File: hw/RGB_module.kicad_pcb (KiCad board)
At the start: 2 copper layers, 30 x 10 mm, 11 parts, among them J1 Conn_01x04, J2 Conn_01x04, J3 Conn_01x03, U1 ZSCS-2016C-08D-Z4

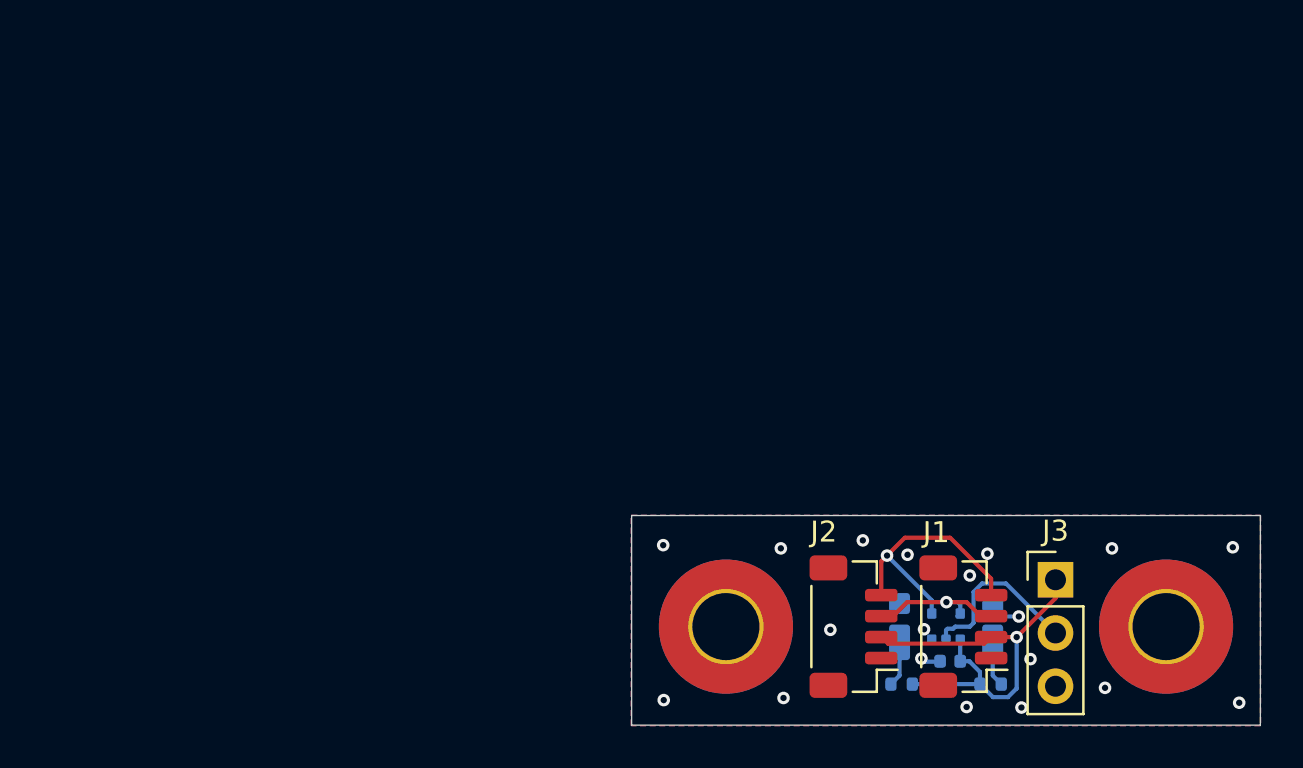
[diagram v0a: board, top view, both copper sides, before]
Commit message: board_v2
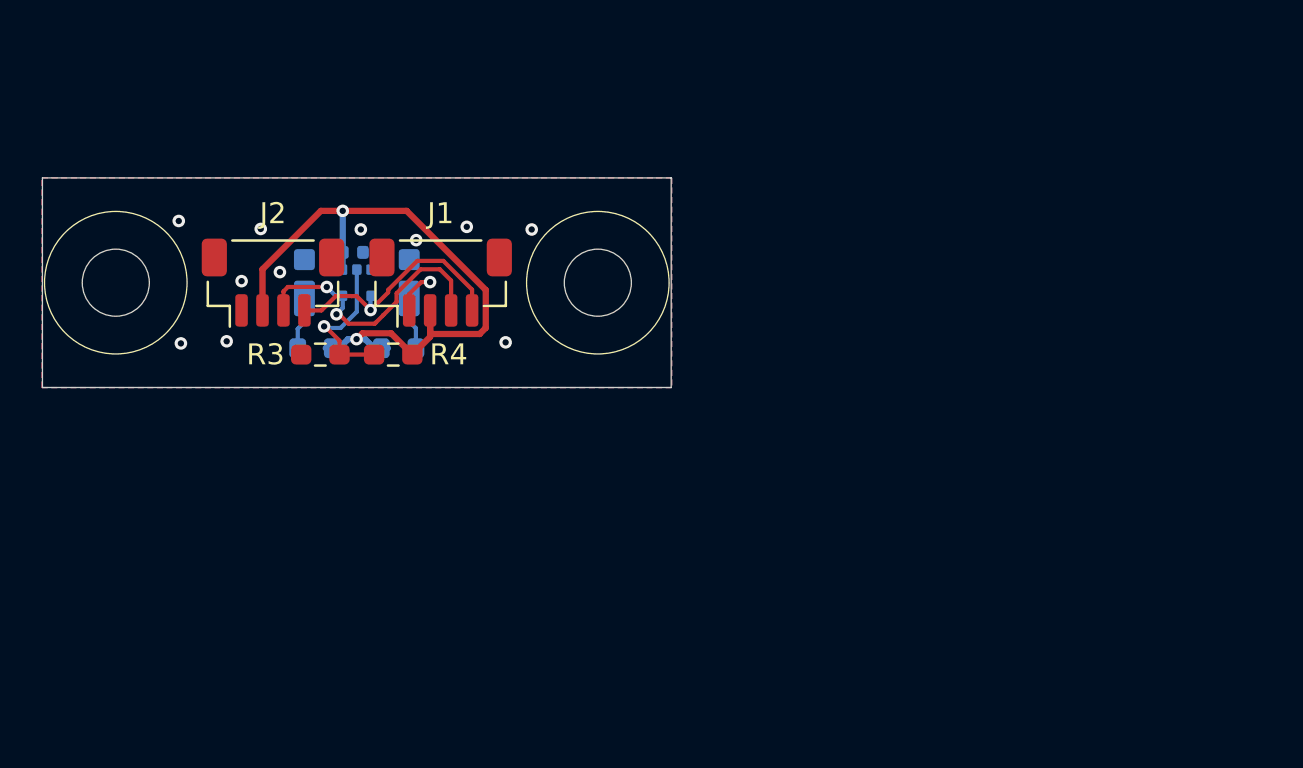
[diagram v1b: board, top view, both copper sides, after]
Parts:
- removed H1, H2: MountingHole, MountingHole:MountingHole_3.2mm_M3_Pad_TopBottom
- removed J3: Conn_01x03, Connector_PinHeader_2.54mm:PinHeader_1x03_P2.54mm_Vertical
- added R3: 0, Resistor_SMD:R_0603_1608Metric_Pad0.98x0.95mm_HandSolder, F.Cu at (45.1, 31.4)
- added R4: 100k, Resistor_SMD:R_0603_1608Metric_Pad0.98x0.95mm_HandSolder, F.Cu at (48.5, 31.4)
- R1, R2: value 8 -> 33; footprint Resistor_SMD:R_0402_1005Metric -> Resistor_SMD:R_0603_1608Metric
- moved C1 34.5 mm to (46.6, 26.5), turned to 0 degrees
- moved D1 32.8 mm to (44.3, 27.9)
- moved U1 32.6 mm to (46.8, 27.9), turned to 90 degrees
- moved R2 32.5 mm to (48.8, 31.1)
- moved D2 32.3 mm to (49.3, 27.9)
- moved R1 32.3 mm to (44.8, 31.1)
- moved J2 32.2 mm to (42.8, 27.9), turned to 0 degrees
- moved J1 29.9 mm to (50.8, 27.9), turned to 0 degrees
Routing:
- net +3.3V: track 20.9 -> 32.8 mm, vias 1 -> 2
- net SDA: track 7.12 -> 13.6 mm, vias 1 -> 2
- net Net-(U1-ADDR): track 8.44 -> 7.26 mm, vias 0 -> 1
- net SCL: track 12.6 -> 11.9 mm
- net GND: track 2.65 -> 2.01 mm, vias 19 -> 12
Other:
- outline, holes or cut-outs redrawn

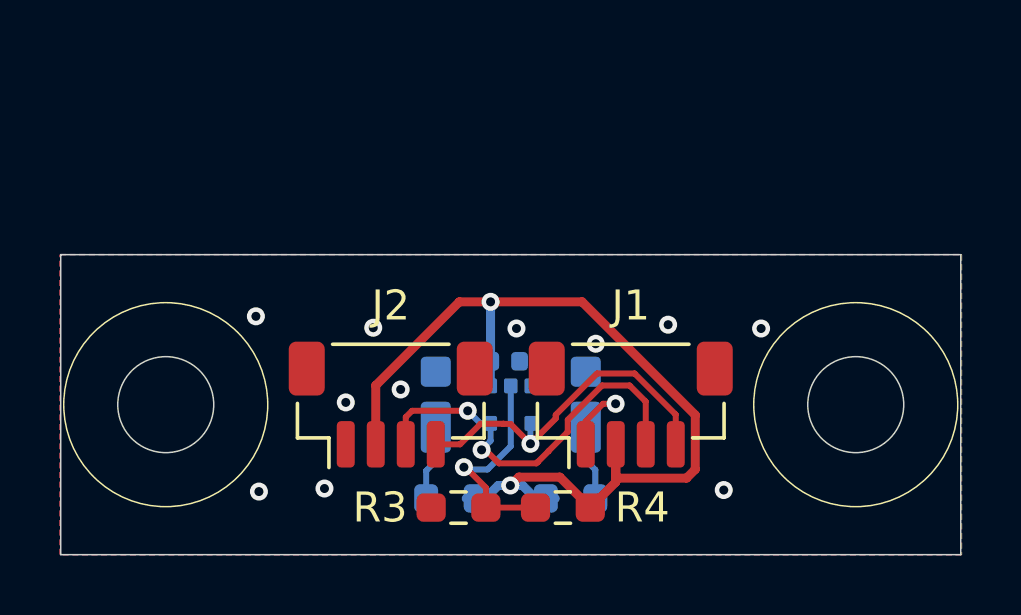
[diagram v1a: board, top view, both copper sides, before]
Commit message: board_v3
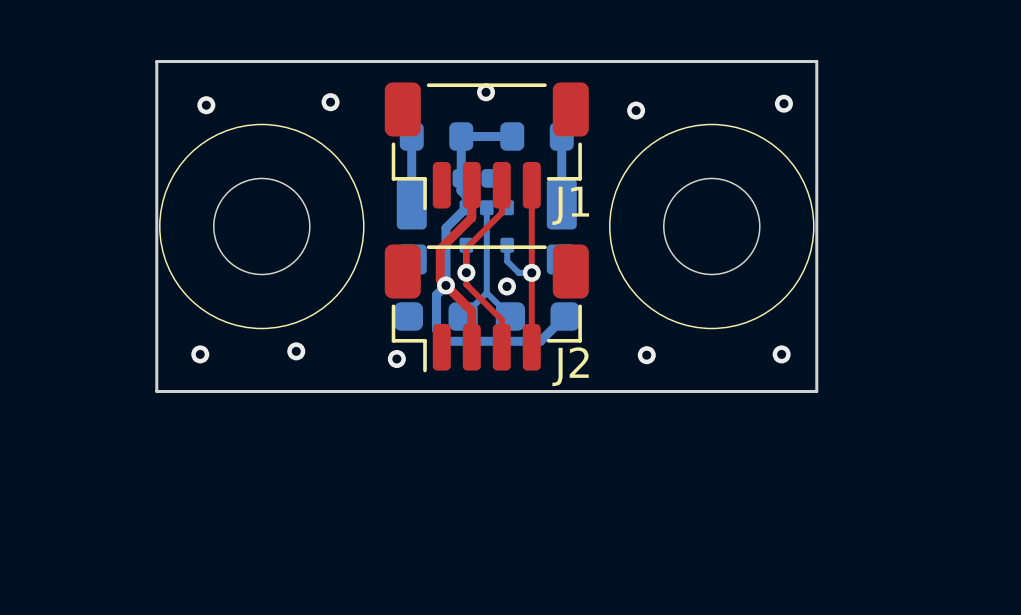
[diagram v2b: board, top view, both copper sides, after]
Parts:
- R3, R4: moved to B.Cu
- moved R2 12.1 mm to (47.7, 19.0)
- moved R1 12.1 mm to (44.3, 19.0)
- moved J1 9.88 mm to (46.0, 19.3)
- moved R4 6.42 mm to (47.7, 25.0)
- moved R3 6.41 mm to (44.3, 25.0)
- moved C1 6.18 mm to (45.6, 20.4)
- moved D1 5.99 mm to (43.5, 22.0), turned to 90 degrees
- moved D2 5.99 mm to (48.5, 22.0), turned to 90 degrees
- moved U1 5.99 mm to (46.0, 22.0)
- moved J2 4.55 mm to (46.0, 24.7)
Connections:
- net SCL renamed Net-(J1-Pin_4)
- net SDA renamed Net-(J1-Pin_3)
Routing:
- net +3.3V: track 32.8 -> 19.7 mm, vias 2 -> 1
- net Net-(J1-Pin_3): track 13.6 -> 7.29 mm, vias 2 -> 1
- net Net-(J1-Pin_4): track 11.9 -> 6.91 mm
- net Net-(U1-ADDR): track 7.26 -> 5.06 mm, vias 1 -> 0
- net GND: track 2.01 -> 0.00 mm, vias 12 -> 11
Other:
- board size 30 x 10 mm -> 22 x 11 mm
